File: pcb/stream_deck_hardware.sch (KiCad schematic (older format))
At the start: 16 parts

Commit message: Schematic update
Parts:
- removed P?: USB_C_Plug, symbol Connector:USB_C_Plug
- added J?: USB_C_Receptacle_USB2.0, Connector_USB:USB_C_Receptacle_Palconn_UTC16-G, symbol Connector:USB_C_Receptacle_USB2.0
- added R? (x4): R, symbol Device:R
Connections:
- net labels added: USB_DM, USB_DP
- wire segments 56 -> 81
- no-connect marks 9 -> 3
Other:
- moved on the sheet: C?

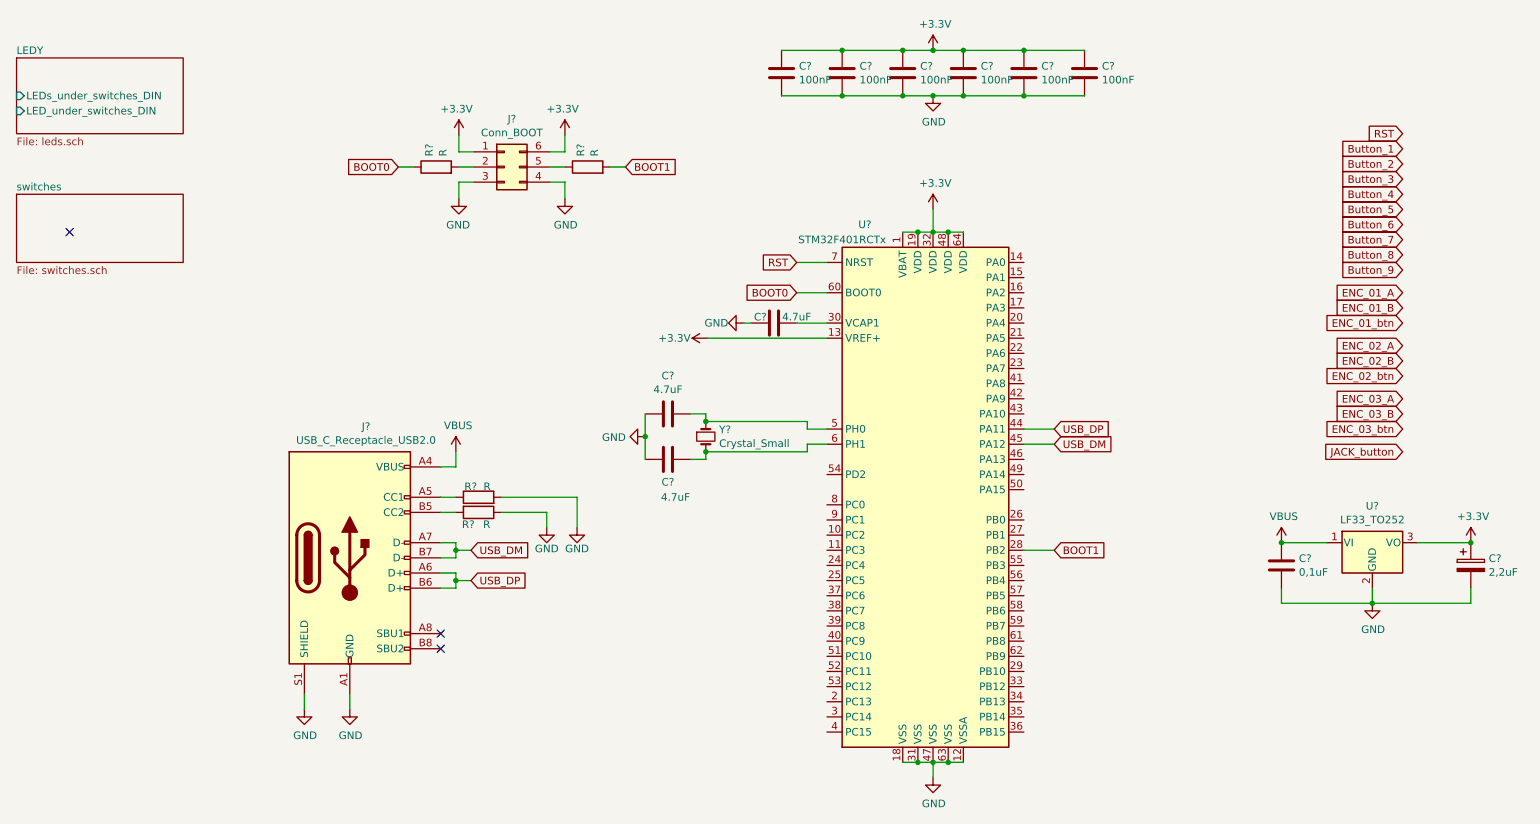
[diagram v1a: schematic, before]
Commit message: Schematic version 1.0
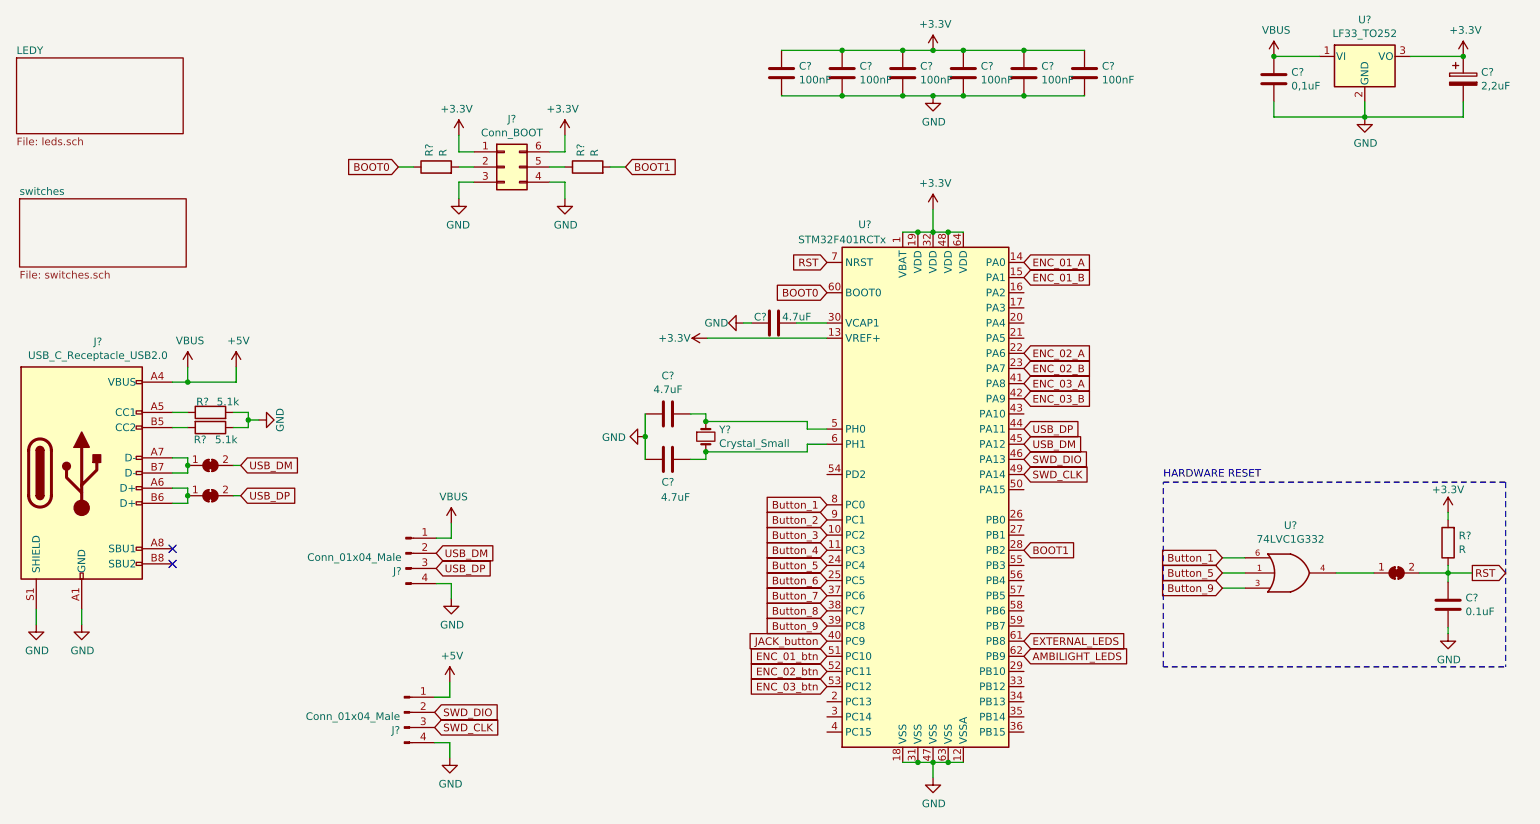
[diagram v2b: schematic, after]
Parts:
- added C?: 0.1uF, symbol Device:C
- added J? (x2): Conn_01x04_Male, symbol Connector:Conn_01x04_Male
- added JP? (x3): SolderJumper_2_Bridged, symbol Jumper:SolderJumper_2_Bridged
- added R?: R, symbol Device:R
- added U?: 74LVC1G332, symbol 74xGxx:74LVC1G332
- R? (x2): value R -> 5.1k
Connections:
- net +3V3: now also R?.2
- net Button_1: now also U?.8 (PC0), U?.6
- net Button_2: now also U?.9 (PC1)
- net Button_3: now also U?.10 (PC2)
- net Button_4: now also U?.11 (PC3)
- net Button_5: now also U?.24 (PC4), U?.1
- net Button_6: now also U?.25 (PC5)
- net Button_7: now also U?.37 (PC6)
- net Button_8: now also U?.38 (PC7)
- net Button_9: now also U?.39 (PC8), U?.3
- net ENC_01_A: now also U?.14 (PA0)
- net ENC_01_B: now also U?.15 (PA1)
- net ENC_01_btn: now also U?.51 (PC10)
- net ENC_02_A: now also U?.22 (PA6)
- net ENC_02_B: now also U?.23 (PA7)
- net ENC_02_btn: now also U?.52 (PC11)
- net ENC_03_A: now also U?.41 (PA8)
- net ENC_03_B: now also U?.42 (PA9)
- net ENC_03_btn: now also U?.53 (PC12)
- net GND: now also C?.2, J?.4 (Pin_4), J?.4 (Pin_4), U?.2 (GND)
- net JACK_button: now also U?.40 (PC9)
- net RST: now also C?.1, JP?.2 (B), R?.1
- net USB_DM: now also J?.2 (Pin_2), JP?.2 (B); no longer J?.A7 (D-), J?.B7 (D-)
- net USB_DP: now also J?.3 (Pin_3), JP?.2 (B); no longer J?.A6 (D+), J?.B6 (D+)
- net SWD_DIO: now reaches U?.46 (PA13)
- net SWD_DIO: now also J?.2 (Pin_2)
- net SWD_CLK: now reaches U?.49 (PA14)
- net SWD_CLK: now also J?.3 (Pin_3)
- net EXTERNAL_LEDS: now reaches U?.61 (PB8)
- net AMBILIGHT_LEDS: now reaches U?.62 (PB9)
- net VBUS renamed +5V
- net +5V: now also J?.1 (Pin_1), J?.1 (Pin_1)
- new net: J?.A6 (D+), J?.B6 (D+), JP?.1 (A)
- new net: J?.A7 (D-), J?.B7 (D-), JP?.1 (A)
- new net: JP?.1 (A), U?.4
- new net VCC: U?.5 (VCC)
- no-connect marks 3 -> 2
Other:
- note added: "HARDWARE RESET\n"
- moved on the sheet: C?, J?, R?, U?
